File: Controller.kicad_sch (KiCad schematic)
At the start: 25 parts, among them IC3 STM32H563VGT6

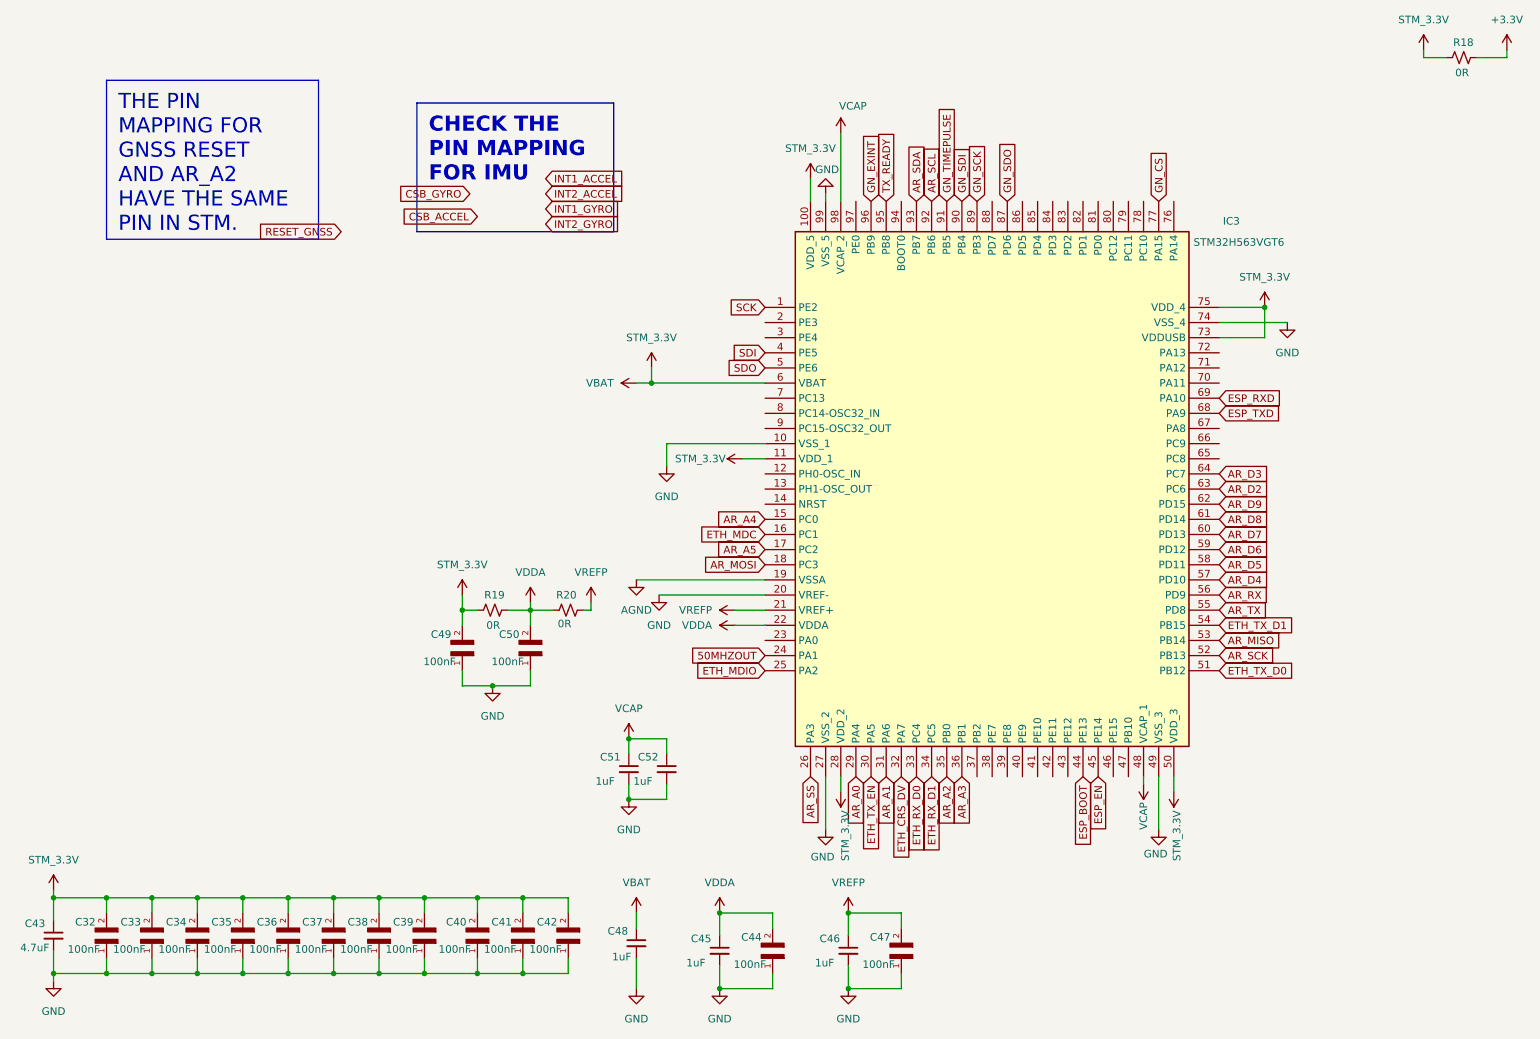
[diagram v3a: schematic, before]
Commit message: new table
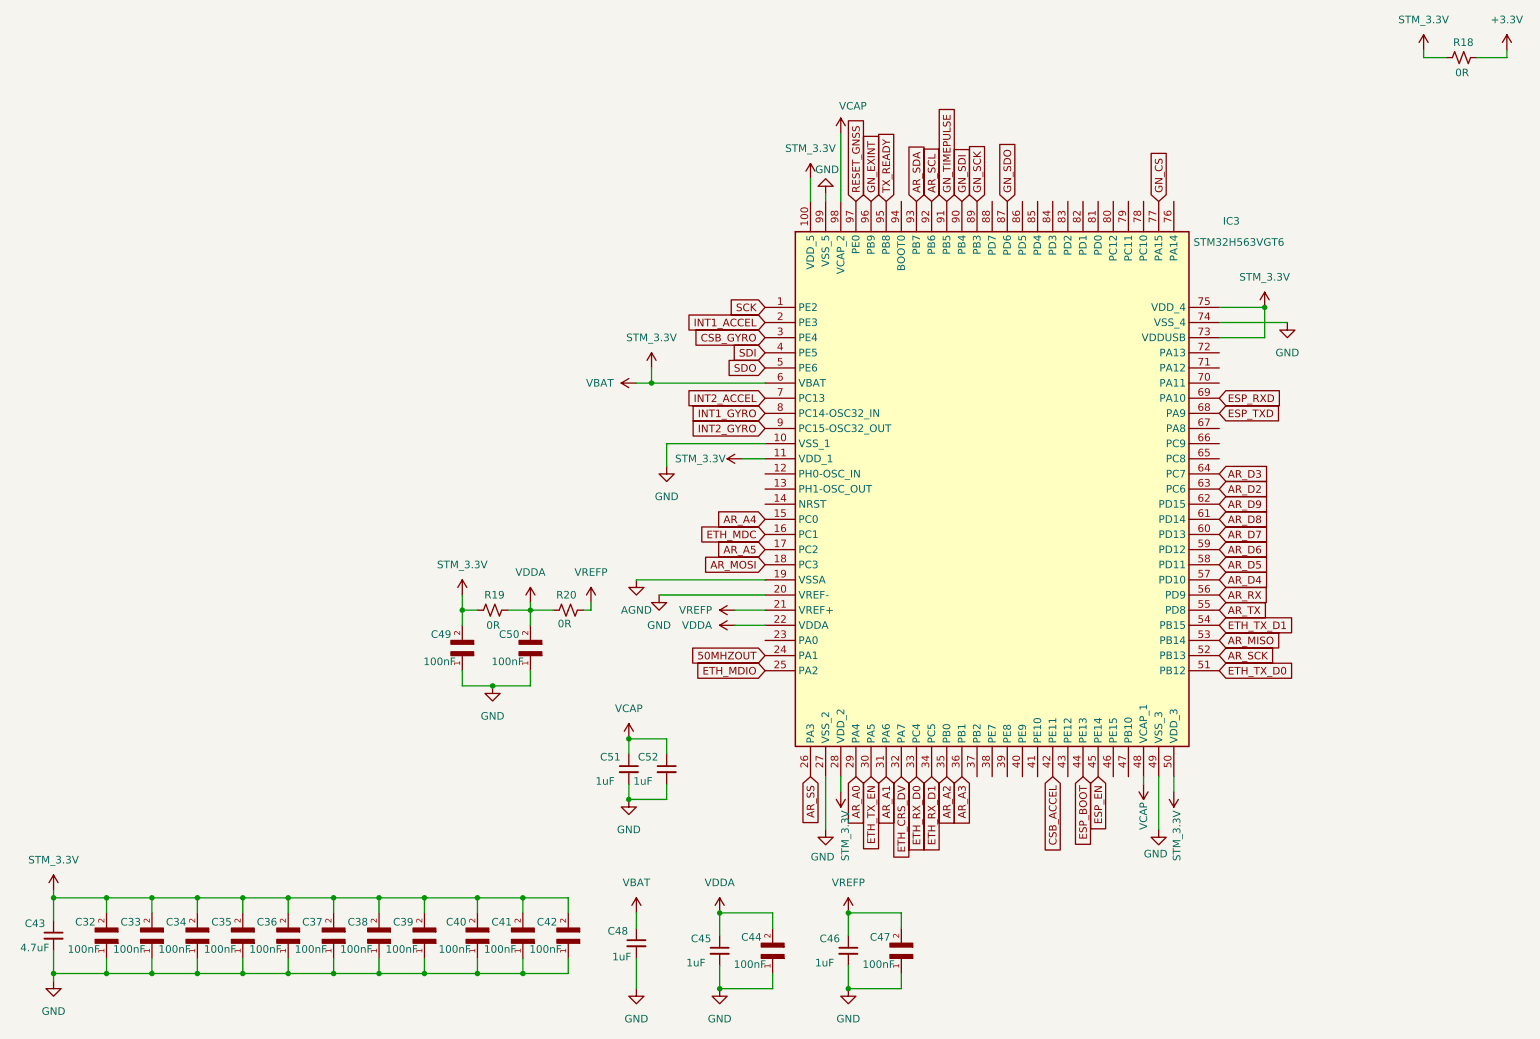
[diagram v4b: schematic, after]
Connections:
- net CSB_ACCEL: now also IC3.42 (PE11)
- net CSB_GYRO: now also IC3.3 (PE4)
- net INT1_ACCEL: now also IC3.2 (PE3)
- net INT1_GYRO: now also IC3.8 (PC14-OSC32_IN)
- net INT2_ACCEL: now also IC3.7 (PC13)
- net INT2_GYRO: now also IC3.9 (PC15-OSC32_OUT)
- net RESET_GNSS: now also IC3.97 (PE0)
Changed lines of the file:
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@@
-		)
-	)
-	(text_box "CHECK THE PIN MAPPING FOR IMU"
-		(exclude_from_sim no)
-		(at 85.09 36.83 0)
-		(size 33.02 21.59)
-		(stroke
-			(width 0)
-			(type default)
-		)
-		(fill
-			(type color)
-			(color 114 255 146 1)
-		)
-		(effects
-			(font
-				(size 2.54 2.54)
-				(thickness 0.254)
-				(bold yes)
-			)
-			(justify left top)
-		)
-	)
-	(text_box "THE PIN MAPPING FOR GNSS RESET AND AR_A2 HAVE THE SAME PIN IN STM."
-		(exclude_from_sim no)
-		(at 33.02 33.02 0)
-		(size 35.56 26.67)
-		(stroke
-			(width 0)
-			(type default)
-		)
-		(fill
-			(type color)
-			(color 140 255 96 1)
-		)
-		(effects
-			(font
-				(size 2.54 2.54)
-			)
-			(justify left top)
 		)
 	)
@@
 	(global_label "INT2_ACCEL"
 		(shape input)
-		(at 106.68 52.07 0)
-		(fields_autoplaced yes)
-		(effects
-			(font
-				(size 1.27 1.27)
-			)
-			(justify left)
-		)
-		(property "Intersheetrefs" "${INTERSHEET_REFS}"
-			(at 120.5509 52.07 0)
-			(effects
-				(font
-					(size 1.27 1.27)
-				)
-				(justify left)
+		(at 143.51 86.36 180)
+		(fields_autoplaced yes)
+		(effects
+			(font
+				(size 1.27 1.27)
+			)
+			(justify right)
+		)
+		(property "Intersheetrefs" "${INTERSHEET_REFS}"
+			(at 129.6391 86.36 0)
+			(effects
+				(font
+					(size 1.27 1.27)
+				)
+				(justify right)
 				(hide yes)
 			)
@@
 	(global_label "INT1_ACCEL"
 		(shape input)
-		(at 106.68 49.53 0)
-		(fields_autoplaced yes)
-		(effects
-			(font
-				(size 1.27 1.27)
-			)
-			(justify left)
-		)
-		(property "Intersheetrefs" "${INTERSHEET_REFS}"
-			(at 120.5509 49.53 0)
-			(effects
-				(font
-					(size 1.27 1.27)
-				)
-				(justify left)
+		(at 143.51 73.66 180)
+		(fields_autoplaced yes)
+		(effects
+			(font
+				(size 1.27 1.27)
+			)
+			(justify right)
+		)
+		(property "Intersheetrefs" "${INTERSHEET_REFS}"
+			(at 129.6391 73.66 0)
+			(effects
+				(font
+					(size 1.27 1.27)
+				)
+				(justify right)
 				(hide yes)
 			)
@@
 	(global_label "INT1_GYRO"
 		(shape input)
-		(at 106.68 54.61 0)
-		(fields_autoplaced yes)
-		(effects
-			(font
-				(size 1.27 1.27)
-			)
-			(justify left)
-		)
-		(property "Intersheetrefs" "${INTERSHEET_REFS}"
-			(at 119.7043 54.61 0)
-			(effects
-				(font
-					(size 1.27 1.27)
-				)
-				(justify left)
+		(at 143.51 88.9 180)
+		(fields_autoplaced yes)
+		(effects
+			(font
+				(size 1.27 1.27)
+			)
+			(justify right)
+		)
+		(property "Intersheetrefs" "${INTERSHEET_REFS}"
+			(at 130.4857 88.9 0)
+			(effects
+				(font
+					(size 1.27 1.27)
+				)
+				(justify right)
 				(hide yes)
 			)
@@
 	(global_label "RESET_GNSS"
 		(shape input)
-		(at 72.39 58.42 180)
-		(fields_autoplaced yes)
-		(effects
-			(font
-				(size 1.27 1.27)
-			)
-			(justify right)
-		)
-		(property "Intersheetrefs" "${INTERSHEET_REFS}"
-			(at 57.6726 58.42 0)
-			(effects
-				(font
-					(size 1.27 1.27)
-				)
-				(justify right)
+		(at 158.75 53.34 90)
+		(fields_autoplaced yes)
+		(effects
+			(font
+				(size 1.27 1.27)
+			)
+			(justify left)
+		)
+		(property "Intersheetrefs" "${INTERSHEET_REFS}"
+			(at 158.75 38.6226 90)
+			(effects
+				(font
+					(size 1.27 1.27)
+				)
+				(justify left)
 				(hide yes)
 			)
@@
 	(global_label "CSB_ACCEL"
 		(shape input)
-		(at 95.25 55.88 180)
-		(fields_autoplaced yes)
-		(effects
-			(font
-				(size 1.27 1.27)
-			)
-			(justify right)
-		)
-		(property "Intersheetrefs" "${INTERSHEET_REFS}"
-			(at 81.742 55.88 0)
+		(at 191.77 149.86 270)
+		(fields_autoplaced yes)
+		(effects
+			(font
+				(size 1.27 1.27)
+			)
+			(justify right)
+		)
+		(property "Intersheetrefs" "${INTERSHEET_REFS}"
+			(at 191.77 163.368 90)
 			(effects
 				(font
@@
 	(global_label "INT2_GYRO"
 		(shape input)
-		(at 106.68 57.15 0)
-		(fields_autoplaced yes)
-		(effects
-			(font
-				(size 1.27 1.27)
-			)
-			(justify left)
-		)
-		(property "Intersheetrefs" "${INTERSHEET_REFS}"
-			(at 119.7043 57.15 0)
-			(effects
-				(font
-					(size 1.27 1.27)
-				)
-				(justify left)
+		(at 143.51 91.44 180)
+		(fields_autoplaced yes)
+		(effects
+			(font
+				(size 1.27 1.27)
+			)
+			(justify right)
+		)
+		(property "Intersheetrefs" "${INTERSHEET_REFS}"
+			(at 130.4857 91.44 0)
+			(effects
+				(font
+					(size 1.27 1.27)
+				)
+				(justify right)
 				(hide yes)
 			)
@@
 	(global_label "CSB_GYRO"
 		(shape input)
-		(at 93.98 52.07 180)
-		(fields_autoplaced yes)
-		(effects
-			(font
-				(size 1.27 1.27)
-			)
-			(justify right)
-		)
-		(property "Intersheetrefs" "${INTERSHEET_REFS}"
-			(at 81.3186 52.07 0)
-			(effects
-				(font
+		(at 143.51 76.2 180)
+		(fields_autoplaced yes)
+		(effects
+			(font
+				(size 1.27 1.27)
+			)
+			(justify right)
+		)
+		(property "Intersheetrefs" "${INTERSHEET_REFS}"
+			(at 130.8486 76.2 0)
+			(effects
+				(font
